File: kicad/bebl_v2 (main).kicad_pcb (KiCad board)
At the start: 2 copper layers, 80 x 24 mm, 64 parts, among them P1 ISP, P11 DRV_LED, P12 CHG_LED, P2 FTDI, P3 LiPo, P4 USB-Micro, P5 Alt_Add, P6 Int1, P7 Int2, P8 DRL_LED, SW1 RST, SW2 MODE, U1 ATMEGA328, U2 FAN5346, U3 ADXL345, U4 MCP73831, U5 TPS61221DCK, X1 8MHz

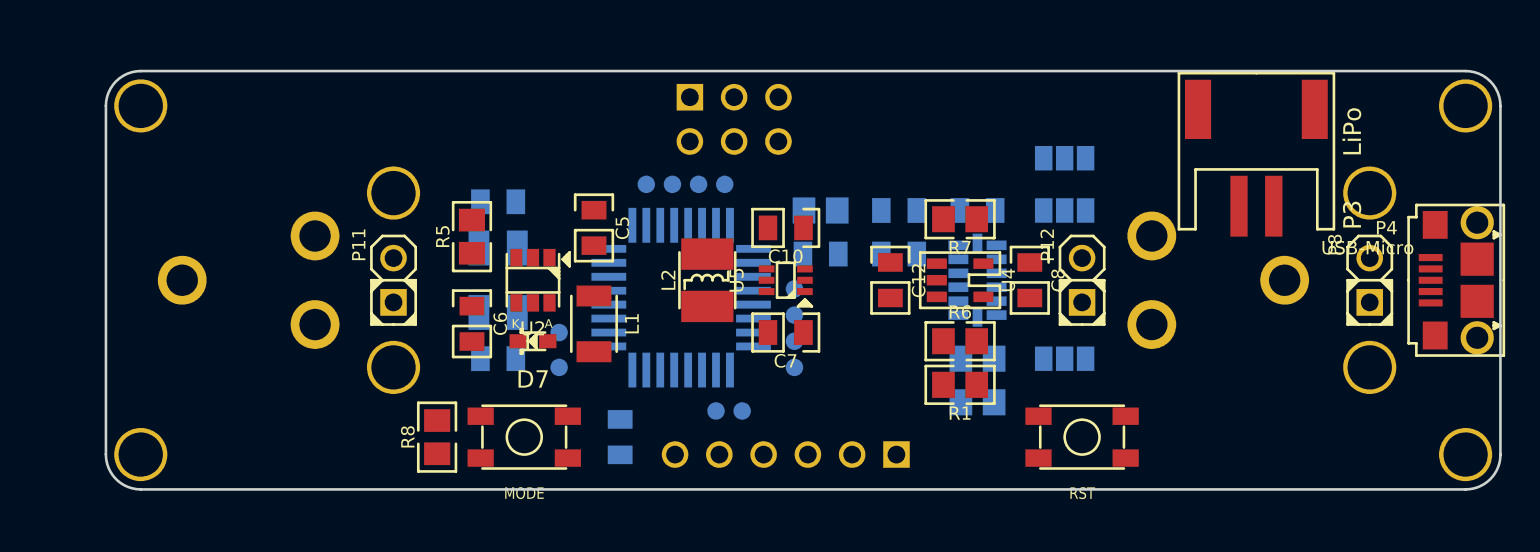
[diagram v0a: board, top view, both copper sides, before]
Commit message: bebl_v2 3d of housing, work in progress
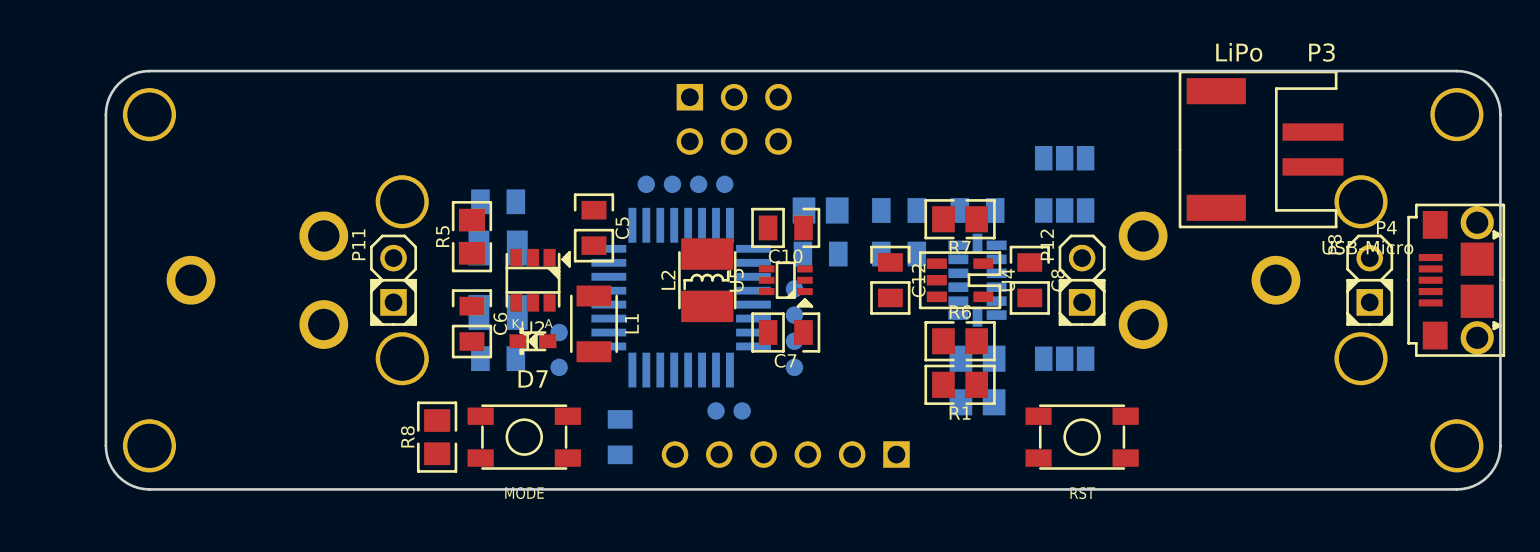
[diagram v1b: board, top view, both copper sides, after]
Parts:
- moved P3 5.66 mm to (100.0, 42.5), turned to 270 degrees
- moved SC1 0.71 mm to (40.5, 59.5)
- moved SC2 0.71 mm to (115.5, 40.5)
- moved SC3 0.71 mm to (115.5, 59.5)
- moved SC4 0.71 mm to (40.5, 40.5)
- moved SC5 0.71 mm to (55.0, 54.5)
- moved SC6 0.71 mm to (55.0, 45.5)
- moved SC7 0.71 mm to (110.0, 45.5)
- moved SC8 0.71 mm to (110.0, 54.5)
- moved B14 0.50 mm to (97.5, 50.0)
- moved B15 0.50 mm to (50.5, 50.0)
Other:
- outline, holes or cut-outs redrawn
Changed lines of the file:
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@@
-(kicad_pcb (version 4) (host pcbnew "(2014-09-25 BZR 5147)-product")
+(kicad_pcb (version 4) (host pcbnew "(2014-jul-16 BZR unknown)-product")
   (general
     (links 133)
     (no_connects 133)
-    (area 37.8537 37.5442 118.521201 63.02209)
+    (area 37.924999 35.7817 118.521201 63.02209)
     (thickness 1.6)
     (drawings 8)
@@
   )
   (module bebl_v2_pretty:batt_clip (layer B.Cu)
-    (at 98 50 180)
+    (at 97.5 50 180)
     (fp_text reference B14 (at 3.556 0 450) (layer B.SilkS)
       (effects (font (size 1.5 1.5) (thickness 0.15)) (justify mirror))
@@
   )
   (module bebl_v2_pretty:batt_clip (layer B.Cu)
-    (at 50 50)
+    (at 50.5 50)
     (fp_text reference B15 (at 3.556 0 270) (layer B.SilkS)
       (effects (font (size 1.5 1.5) (thickness 0.15)) (justify mirror))
@@
   )
   (module bebl_v2_pretty:screw_3mm (layer F.Cu)
-    (at 110.5 55)
+    (at 110 54.5)
     (descr "vite 2,5mm")
     (fp_text reference SC8 (at 0 1.0795) (layer F.SilkS) hide
@@
   )
   (module bebl_v2_pretty:screw_3mm (layer F.Cu)
-    (at 110.5 45)
+    (at 110 45.5)
     (descr "vite 2,5mm")
     (fp_text reference SC7 (at 0 1.0795) (layer F.SilkS) hide
@@
   )
   (module bebl_v2_pretty:screw_3mm (layer F.Cu)
-    (at 54.5 45)
+    (at 55 45.5)
     (descr "vite 2,5mm")
     (fp_text reference SC6 (at 0 1.0795) (layer F.SilkS) hide
@@
   )
   (module bebl_v2_pretty:screw_3mm (layer F.Cu)
-    (at 54.5 55)
+    (at 55 54.5)
     (descr "vite 2,5mm")
     (fp_text reference SC5 (at 0 1.0795) (layer F.SilkS) hide
@@
   )
   (module bebl_v2_pretty:screw_3mm (layer F.Cu)
-    (at 40 60)
+    (at 40.5 59.5)
     (descr "vite 2,5mm")
     (fp_text reference SC1 (at 0 1.0795) (layer F.SilkS) hide
@@
   )
   (module bebl_v2_pretty:screw_3mm (layer F.Cu)
-    (at 116 40)
+    (at 115.5 40.5)
     (descr "vite 2,5mm")
     (fp_text reference SC2 (at 0 1.0795) (layer F.SilkS) hide
@@
   )
   (module bebl_v2_pretty:screw_3mm (layer F.Cu)
-    (at 116 60)
+    (at 115.5 59.5)
     (descr "vite 2,5mm")
     (fp_text reference SC3 (at 0 1.0795) (layer F.SilkS) hide
@@
   )
   (module bebl_v2_pretty:screw_3mm (layer F.Cu)
-    (at 40 40)
+    (at 40.5 40.5)
     (descr "vite 2,5mm")
     (fp_text reference SC4 (at 0 1.0795) (layer F.SilkS) hide
@@
   )
   (module bebl_v2_pretty:CONN_JST-2_SMD (layer F.Cu)
-    (at 104 38.5 180)
+    (at 100 42.5 270)
     (tags JST)
-    (fp_text reference P3 (at -5.5245 -7.747 450) (layer F.SilkS)
+    (fp_text reference P3 (at -5.5245 -7.747 540) (layer F.SilkS)
       (effects (font (size 1.016 1.016) (thickness 0.1524)))
     )
-    (fp_text value LiPo (at -5.5245 -2.9845 450) (layer F.SilkS)
+    (fp_text value LiPo (at -5.5245 -2.9845 540) (layer F.SilkS)
       (effects (font (size 1.016 1.016) (thickness 0.1524)))
     )
@@
     (fp_line (start 3.4925 -8.5725) (end 4.445 -8.5725) (layer F.SilkS) (width 0.1524))
     (fp_line (start 4.445 0.381) (end 0 0.381) (layer F.SilkS) (width 0.1524))
-    (pad "" smd rect (at -3.34772 -1.69926 180) (size 1.4986 3.39598) (layers F.Cu F.Paste F.Mask))
-    (pad 1 smd rect (at -0.99822 -7.24916 180) (size 0.99568 3.49758) (layers F.Cu F.Paste F.Mask)
+    (pad "" smd rect (at -3.34772 -1.69926 270) (size 1.4986 3.39598) (layers F.Cu F.Paste F.Mask))
+    (pad 1 smd rect (at -0.99822 -7.24916 270) (size 0.99568 3.49758) (layers F.Cu F.Paste F.Mask)
       (net 13 /BAT))
-    (pad 2 smd rect (at 0.99822 -7.24916 180) (size 0.99568 3.49758) (layers F.Cu F.Paste F.Mask)
-      (net 14 GND))
-    (pad "" smd rect (at 3.34772 -1.69926 180) (size 1.4986 3.39598) (layers F.Cu F.Paste F.Mask))
+    (pad 2 smd rect (at 0.99822 -7.24916 270) (size 0.99568 3.49758) (layers F.Cu F.Paste F.Mask)
+      (net 14 GND))
+    (pad "" smd rect (at 3.34772 -1.69926 270) (size 1.4986 3.39598) (layers F.Cu F.Paste F.Mask))
     (model /home/samata/projects-git/bebl_v2/kicad/3d_modules/s2b-ph-sm4-tb.wrl
       (at (xyz 0 0.254 0))
@@
     )
   )
-  (gr_line (start 38 60) (end 38 40) (angle 90) (layer Edge.Cuts) (width 0.15))
-  (gr_line (start 116 62) (end 40 62) (angle 90) (layer Edge.Cuts) (width 0.15))
-  (gr_line (start 118 40) (end 118 60) (angle 90) (layer Edge.Cuts) (width 0.15))
-  (gr_line (start 40 38) (end 116 38) (angle 90) (layer Edge.Cuts) (width 0.15))
-  (gr_arc (start 40 40) (end 38 40) (angle 90) (layer Edge.Cuts) (width 0.15))
-  (gr_arc (start 40 60) (end 40 62) (angle 90) (layer Edge.Cuts) (width 0.15))
-  (gr_arc (start 116 60) (end 118 60) (angle 90) (layer Edge.Cuts) (width 0.15))
-  (gr_arc (start 116 40) (end 116 38) (angle 90) (layer Edge.Cuts) (width 0.15))
+  (gr_line (start 38 59.5) (end 38 40.5) (angle 90) (layer Edge.Cuts) (width 0.15))
+  (gr_line (start 115.5 62) (end 40.5 62) (angle 90) (layer Edge.Cuts) (width 0.15))
+  (gr_line (start 118 40.5) (end 118 59.5) (angle 90) (layer Edge.Cuts) (width 0.15))
+  (gr_line (start 40.5 38) (end 115.5 38) (angle 90) (layer Edge.Cuts) (width 0.15))
+  (gr_arc (start 40.5 40.5) (end 38 40.5) (angle 90) (layer Edge.Cuts) (width 0.15))
+  (gr_arc (start 40.5 59.5) (end 40.5 62) (angle 90) (layer Edge.Cuts) (width 0.15))
+  (gr_arc (start 115.5 59.5) (end 118 59.5) (angle 90) (layer Edge.Cuts) (width 0.15))
+  (gr_arc (start 115.5 40.5) (end 115.5 38) (angle 90) (layer Edge.Cuts) (width 0.15))
 )

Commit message: working on case for bebl_v2
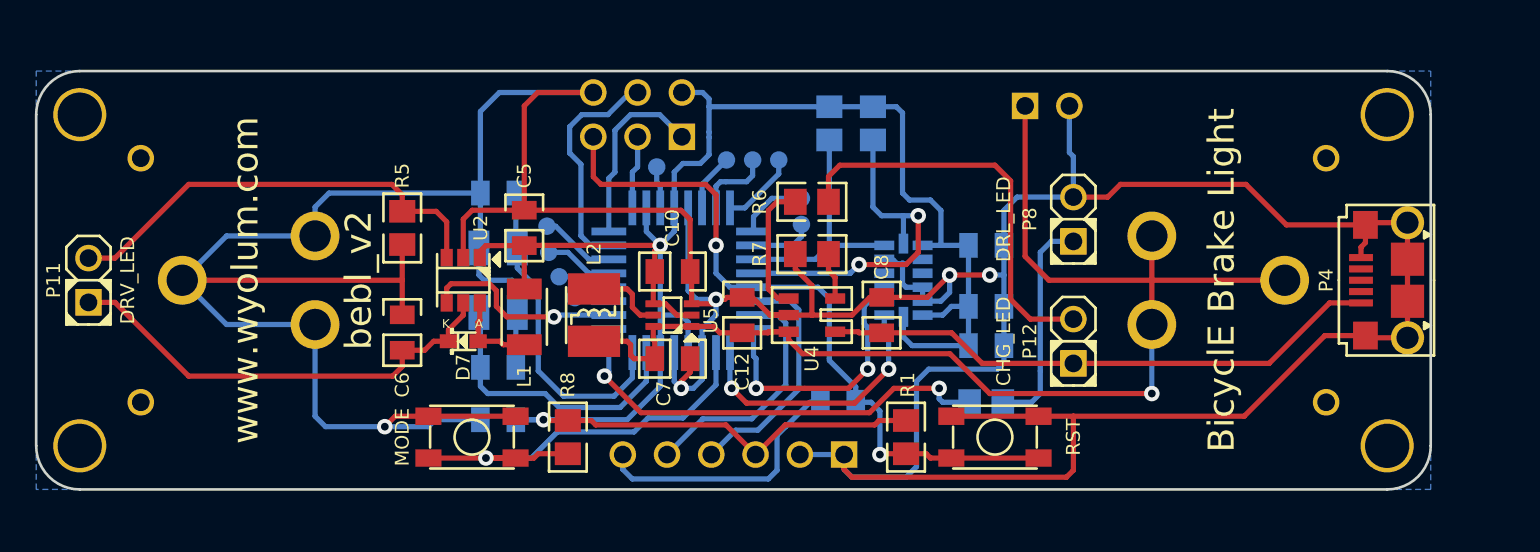
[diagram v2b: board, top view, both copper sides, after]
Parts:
- removed B8, B9: I/O, bebl_v2_pretty:breakout_smd
- removed P5: Alt_Add, bebl_v2_pretty:solder_bridge_3
- removed P6: Int1, bebl_v2_pretty:solder_bridge_3
- removed P7: Int2, bebl_v2_pretty:solder_bridge_3
- P3: value LiPo -> Ext_LiPo; footprint bebl_v2_pretty:CONN_JST-2_SMD -> bebl_v2_pretty:pin_strip_2; moved to B.Cu
- moved C3 20.8 mm to (60.5, 58.0), turned to 0 degrees
- moved R2 18.1 mm to (79.5, 41.0), turned to 90 degrees
- moved P11 17.5 mm to (37.0, 50.0)
- moved P8 17.4 mm to (93.5, 46.5)
- moved SC5 15.2 mm to (40.0, 57.0)
- moved SC6 15.2 mm to (40.0, 43.0)
- moved R3 14.8 mm to (82.0, 41.0), turned to 90 degrees
- moved R4 14.5 mm to (88.5, 57.0)
- moved B3 12.7 mm to (77.9, 45.3)
- moved C4 12.7 mm to (80.0, 57.0), turned to 180 degrees
- moved B2 11.9 mm to (76.6, 43.1)
- moved B4 11.8 mm to (77.9, 46.8)
- moved R6 11.7 mm to (78.5, 45.5)
- moved B1 10.7 mm to (75.1, 43.1)
- moved B5 10.6 mm to (69.6, 43.5)
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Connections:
- C5 pad 1: /VLED -> +3.3V
- L1 pad 1: /VLED -> +3.3V
- P4 pad 2: Net-(P4-Pad2) -> (no net)
- P4 pad 3: Net-(P4-Pad3) -> (no net)
- P4 pad 4: Net-(P4-Pad4) -> (no net)
- R8 pad 2: /INT0 -> /MODE
- SW2 pad 2: /INT0 -> /MODE
- U1 pad 1: Net-(B8-Pad1) -> /ACL_INT1
- U1 pad 2: Net-(B9-Pad1) -> /MODE
- U1 pad 32: /INT0 -> /ACL_INT2
- U2 pad 1: /VLED -> +3.3V
- U3 pad 10: Net-(U3-Pad10) -> (no net)
- U3 pad 11: Net-(U3-Pad11) -> (no net)
- U3 pad 12: /ACL_SDO -> GND
- U3 pad 3: Net-(U3-Pad3) -> (no net)
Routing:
- net GND: track 0.00 -> 283.8 mm, vias 0 -> 5
- net +3.3V: track 0.00 -> 115.3 mm, vias 0 -> 2
- net /BAT: track 0.00 -> 72.4 mm, vias 0 -> 1
- net /RESET: track 0.00 -> 41.3 mm, vias 0 -> 2
- net /VUSB: track 0.00 -> 32.4 mm
- net /MODE: track 0.00 -> 26.6 mm, vias 0 -> 1
- net /LED_A: track 0.00 -> 26.4 mm
- net /DRL_PWM: track 0.00 -> 25.9 mm, vias 0 -> 2
- net /LED_K: track 0.00 -> 25.8 mm
- net Net-(P12-Pad2): track 0.00 -> 23.4 mm
- net /SCL: track 0.00 -> 20.3 mm, vias 0 -> 2
- net /PB7: track 0.00 -> 18.6 mm
- net /PB6: track 0.00 -> 16.6 mm
- net /ACL_INT1: track 0.00 -> 15.5 mm, vias 0 -> 2
- net Net-(C4-Pad1): track 0.00 -> 15.4 mm
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- added copper zone on B.Cu, net GND
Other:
- net class 0.2mm added: clearance 0.2, trace_width 0.2, via_dia 0.889, via_drill 0.635
- net class Default: clearance 0.254 -> 0.25; trace_width 0.254 -> 0.3
- rule trace_clearance: 0.254 -> 0.25
- rule trace_min: 0.254 -> 0.2
- board text added: "(3V3)"
- board text added: "BLK"
- board text added: "BicyclE Brake Light"
- board text added: "GRN"
- board text added: "[+ -]"
- board text added: "[+]"
- board text added: "[-]"
- board text added: "bebl_v2"
- board text added: "www.wyolum.com"
